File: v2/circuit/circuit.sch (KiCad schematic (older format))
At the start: 36 parts, among them J1 Conn_01x05, J2 LEDS, M1 Stepper_Motor_bipolar, SW1 SW_Push, SW2 SW_Push, U1 ATmega328P-AU, U2 4N25, U3 HT1621B, U4 TSR_1-2450, U5 VIM-878, U6 L293D, Y1 Crystal

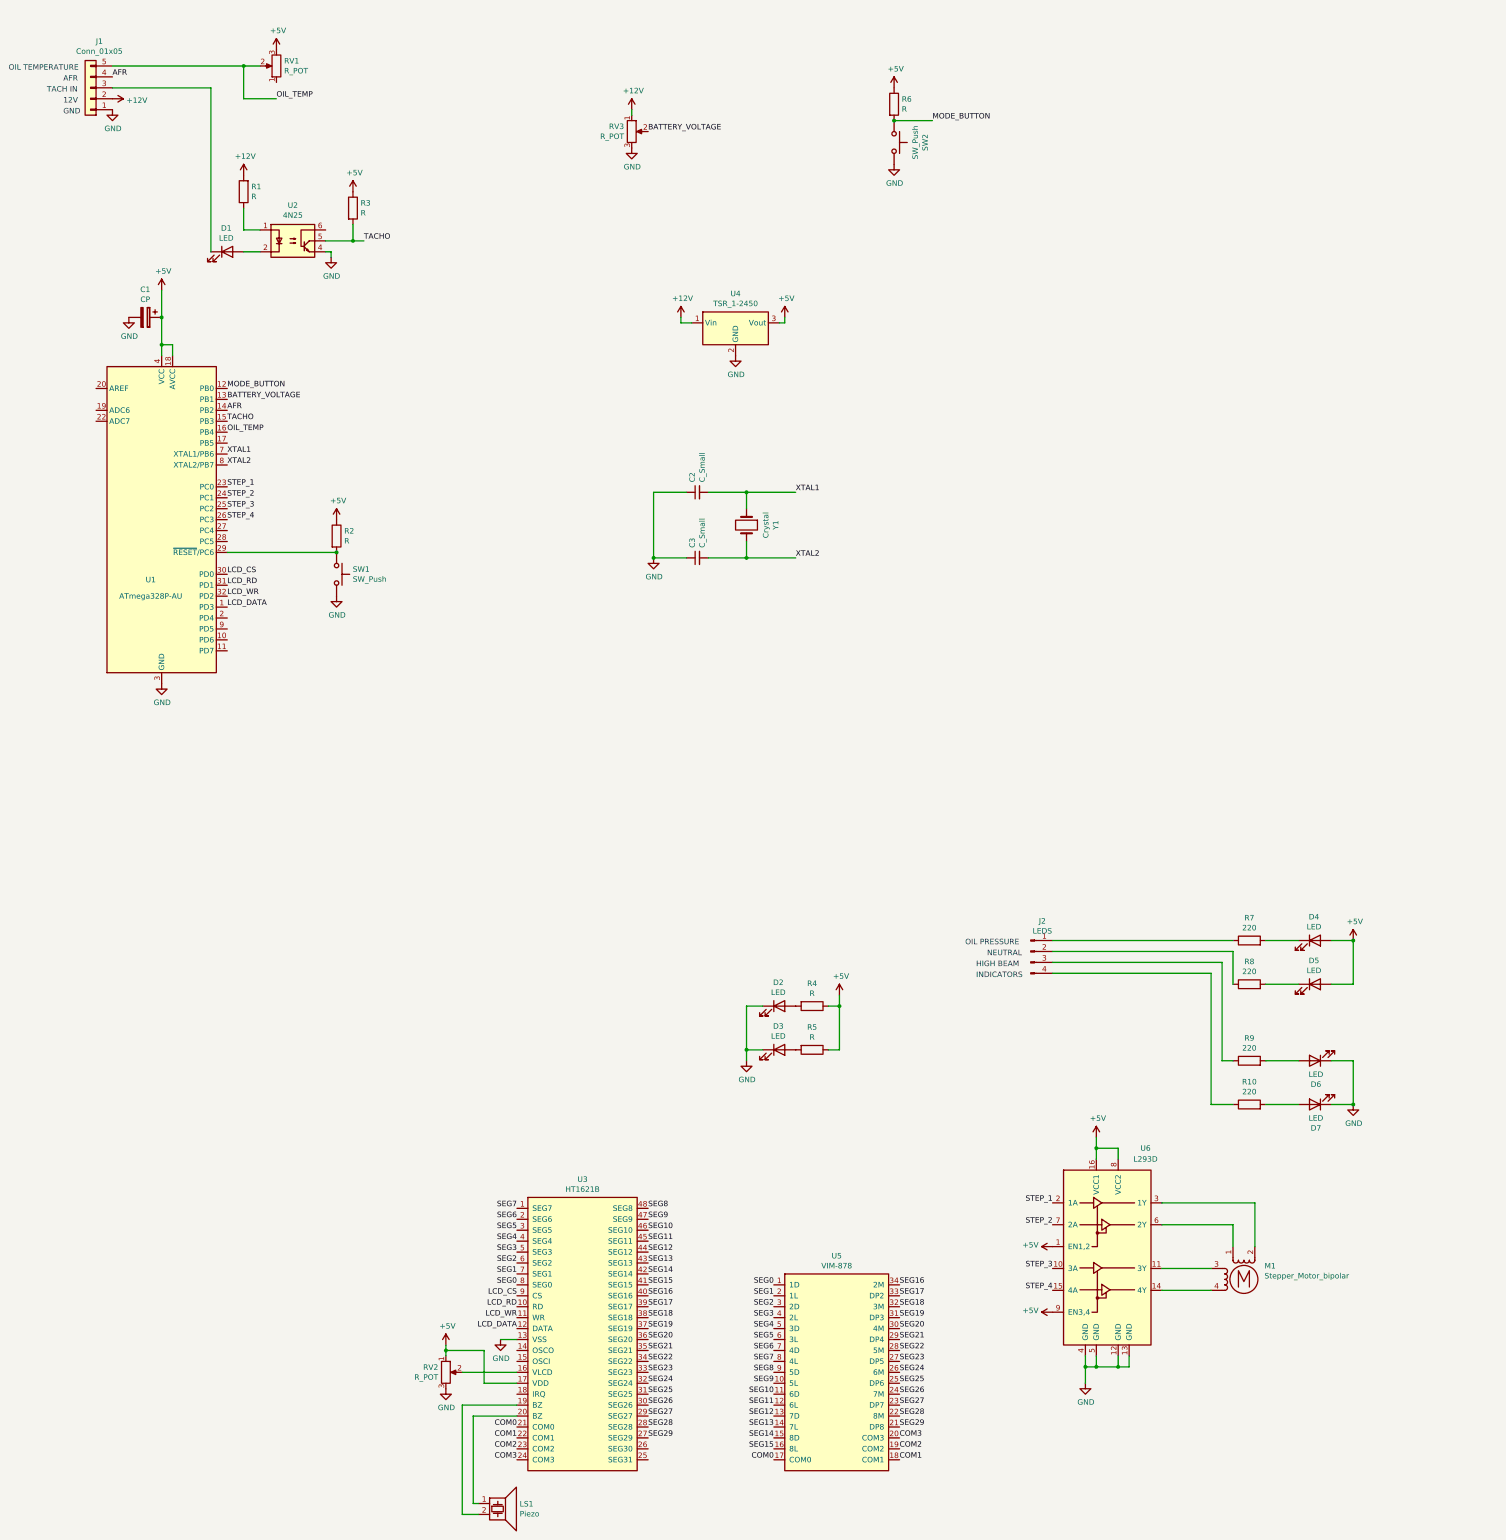
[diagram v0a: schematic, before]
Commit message: Stuff
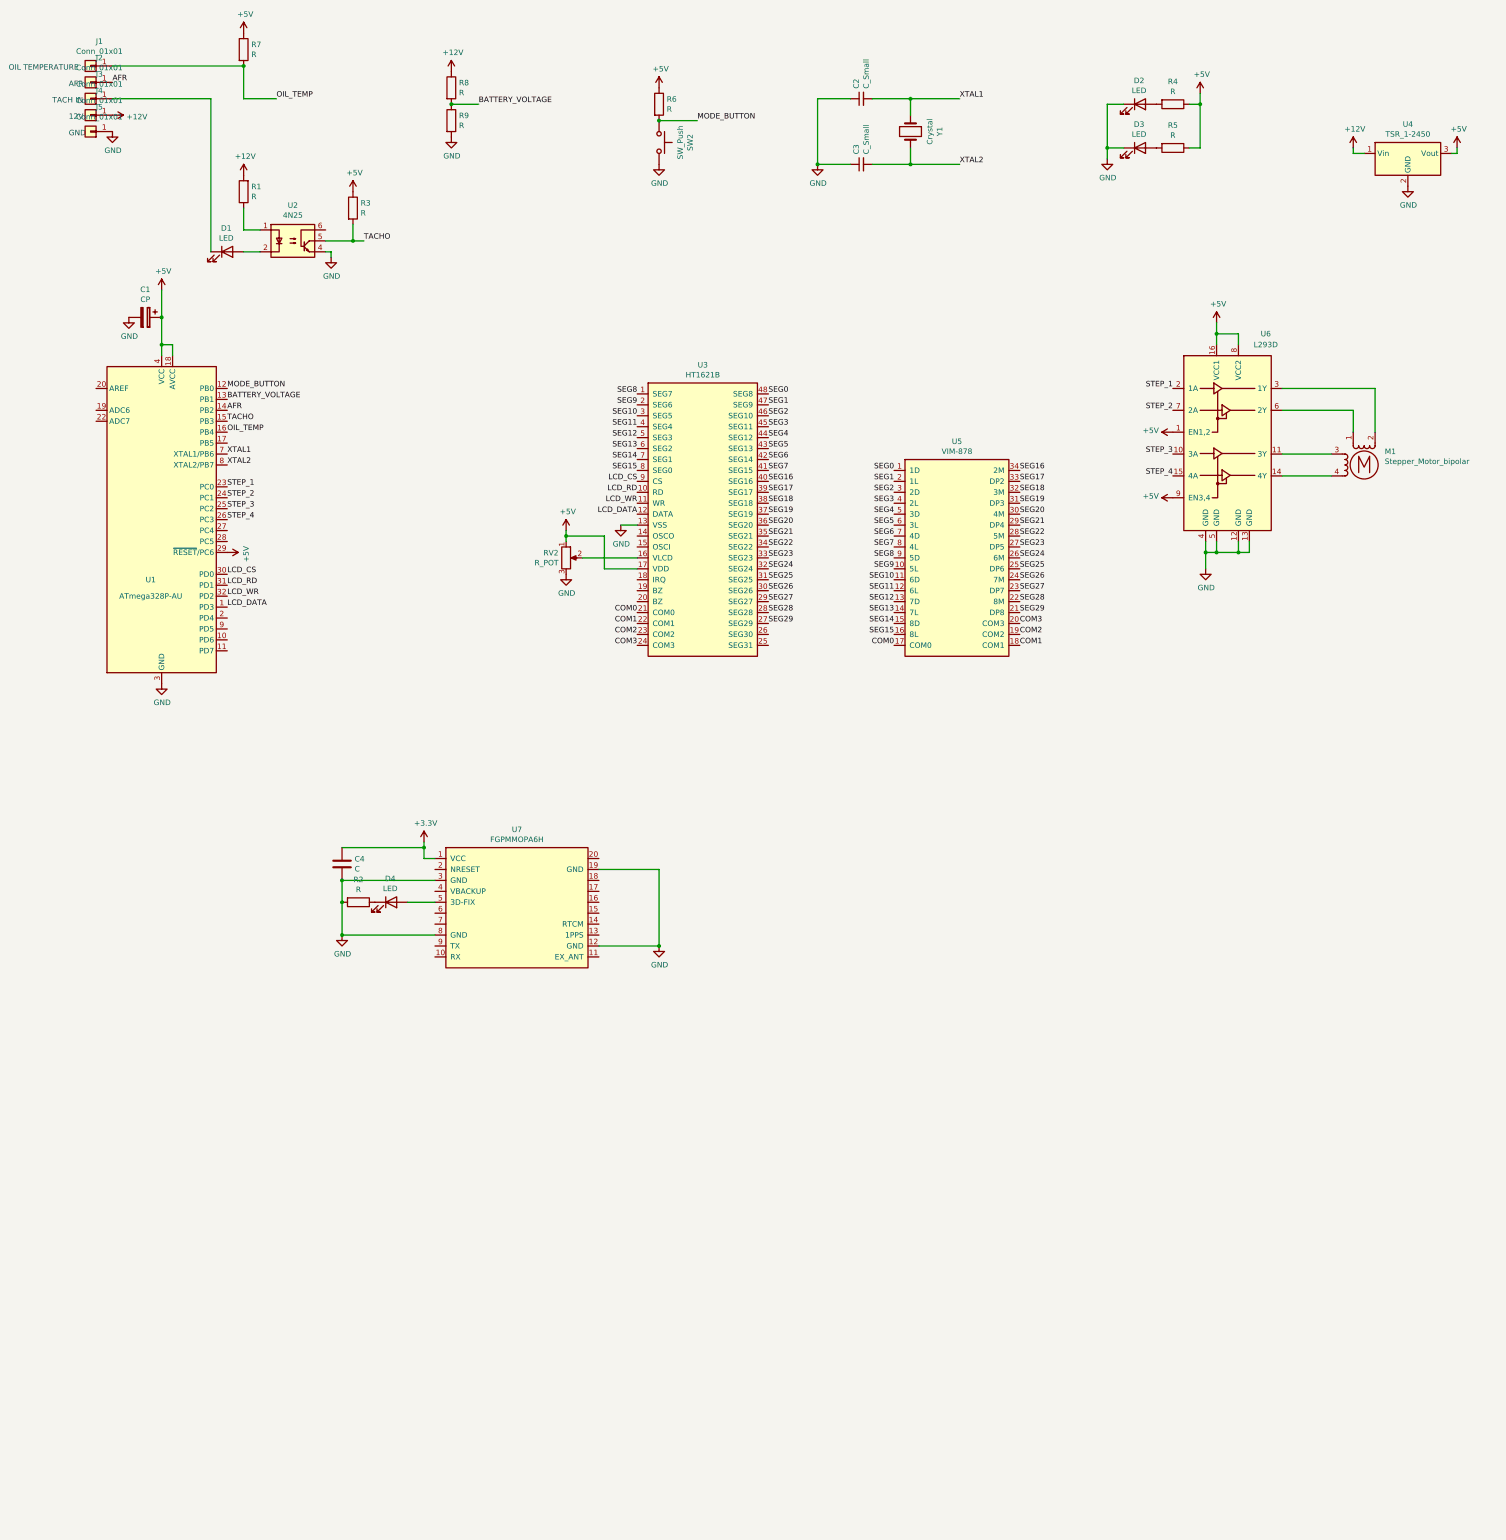
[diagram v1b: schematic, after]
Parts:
- removed D5, D6, D7: LED, LED_SMD:LED_0805_2012Metric, symbol Device:LED
- removed J1: Conn_01x05, Connector_Molex:Molex_PicoBlade_53047-1010_1x05_P1.25mm_Vertical, symbol Connector_Generic:Conn_01x05
- removed J2: LEDS, Connector_PinHeader_2.54mm:PinHeader_1x04_P2.54mm_Vertical, symbol Connector:Conn_01x04_Male
- removed LS1: Piezo, Fuse:Fuse_0201_0603Metric, symbol Device:Speaker_Crystal
- removed R10: 220, Resistor_SMD:R_0805_2012Metric, symbol Device:R
- removed RV1, RV3: R_POT, Potentiometer_THT:Potentiometer_Bourns_3266Y_Vertical, symbol Device:R_POT
- removed SW1: SW_Push, Button_Switch_SMD:SW_SPST_B3S-1000, symbol Switch:SW_Push
- added C4: C, Capacitor_THT:C_Disc_D3.0mm_W2.0mm_P2.50mm, symbol Device:C
- added J1, J2, J3, J4, J5: Conn_01x01, footprints:wire-pad, symbol Connector_Generic:Conn_01x01
- added U7: FGPMMOPA6H, footprints:FGPMMOPA6H, symbol symbol_library:FGPMMOPA6H
- R7, R8, R9: value 220 -> R
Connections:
- net +12V: now also R8.1, J4.1 (Pin_1)
- net +5V: now also R7.1, U1.29 (~RESET~/PC6); no longer D4.2 (A), R2.1
- net AFR: now also J2.1 (Pin_1)
- net BATTERY_VOLTAGE: now also R8.2, R9.1
- net GND: now also R2.2, R9.2, C4.2, J5.1 (Pin_1), U7.12 (GND), U7.19 (GND), U7.3 (GND), U7.8 (GND)
- net OIL_TEMP: now also R7.2, J1.1 (Pin_1)
- net SEG0: now also U3.48 (SEG8); no longer U3.8 (SEG0)
- net SEG1: now also U3.47 (SEG9); no longer U3.7 (SEG1)
- net SEG10: now also U3.3 (SEG5); no longer U3.46 (SEG10)
- net SEG11: now also U3.4 (SEG4); no longer U3.45 (SEG11)
- net SEG12: now also U3.5 (SEG3); no longer U3.44 (SEG12)
- net SEG13: now also U3.6 (SEG2); no longer U3.43 (SEG13)
- net SEG14: now also U3.7 (SEG1); no longer U3.42 (SEG14)
- net SEG15: now also U3.8 (SEG0); no longer U3.41 (SEG15)
- net SEG2: now also U3.46 (SEG10); no longer U3.6 (SEG2)
- net SEG3: now also U3.45 (SEG11); no longer U3.5 (SEG3)
- net SEG4: now also U3.44 (SEG12); no longer U3.4 (SEG4)
- net SEG5: now also U3.43 (SEG13); no longer U3.3 (SEG5)
- net SEG6: now also U3.42 (SEG14); no longer U3.2 (SEG6)
- net SEG7: now also U3.41 (SEG15); no longer U3.1 (SEG7)
- net SEG8: now also U3.1 (SEG7); no longer U3.48 (SEG8)
- net SEG9: now also U3.2 (SEG6); no longer U3.47 (SEG9)
- net at D4.1 (K): now also R2.1; no longer R7.2
- net at D1.1 (K): now also J3.1 (Pin_1)
- new net: D4.2 (A), U7.5 (3D-FIX)
- new net +3V3: C4.1, U7.1 (VCC)
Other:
- note removed: "HIGH BEAM"
- note removed: "INDICATORS"
- note removed: "NEUTRAL"
- note removed: "OIL PRESSURE"
- moved on the sheet: C2, C3, D2, D3, M1, R4, R5, R6, RV2, SW2, U3, U4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
